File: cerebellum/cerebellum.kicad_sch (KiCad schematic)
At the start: 25 parts, among them J1 GPIO, J2 Conn_MOTA, J3 Conn_MOTB, J4 MD_POW, J5 Conn_SPI, J6 Conn_UART, J7 Conn_I2C, J8 VBUS(OUT), J9 3V3(OUT), SW1 PULLUP, SW2 PULLDOWN, SW3 SW_SPDT, U2 POLOLU_TB6612_CARRIER, U3 HC-SR04

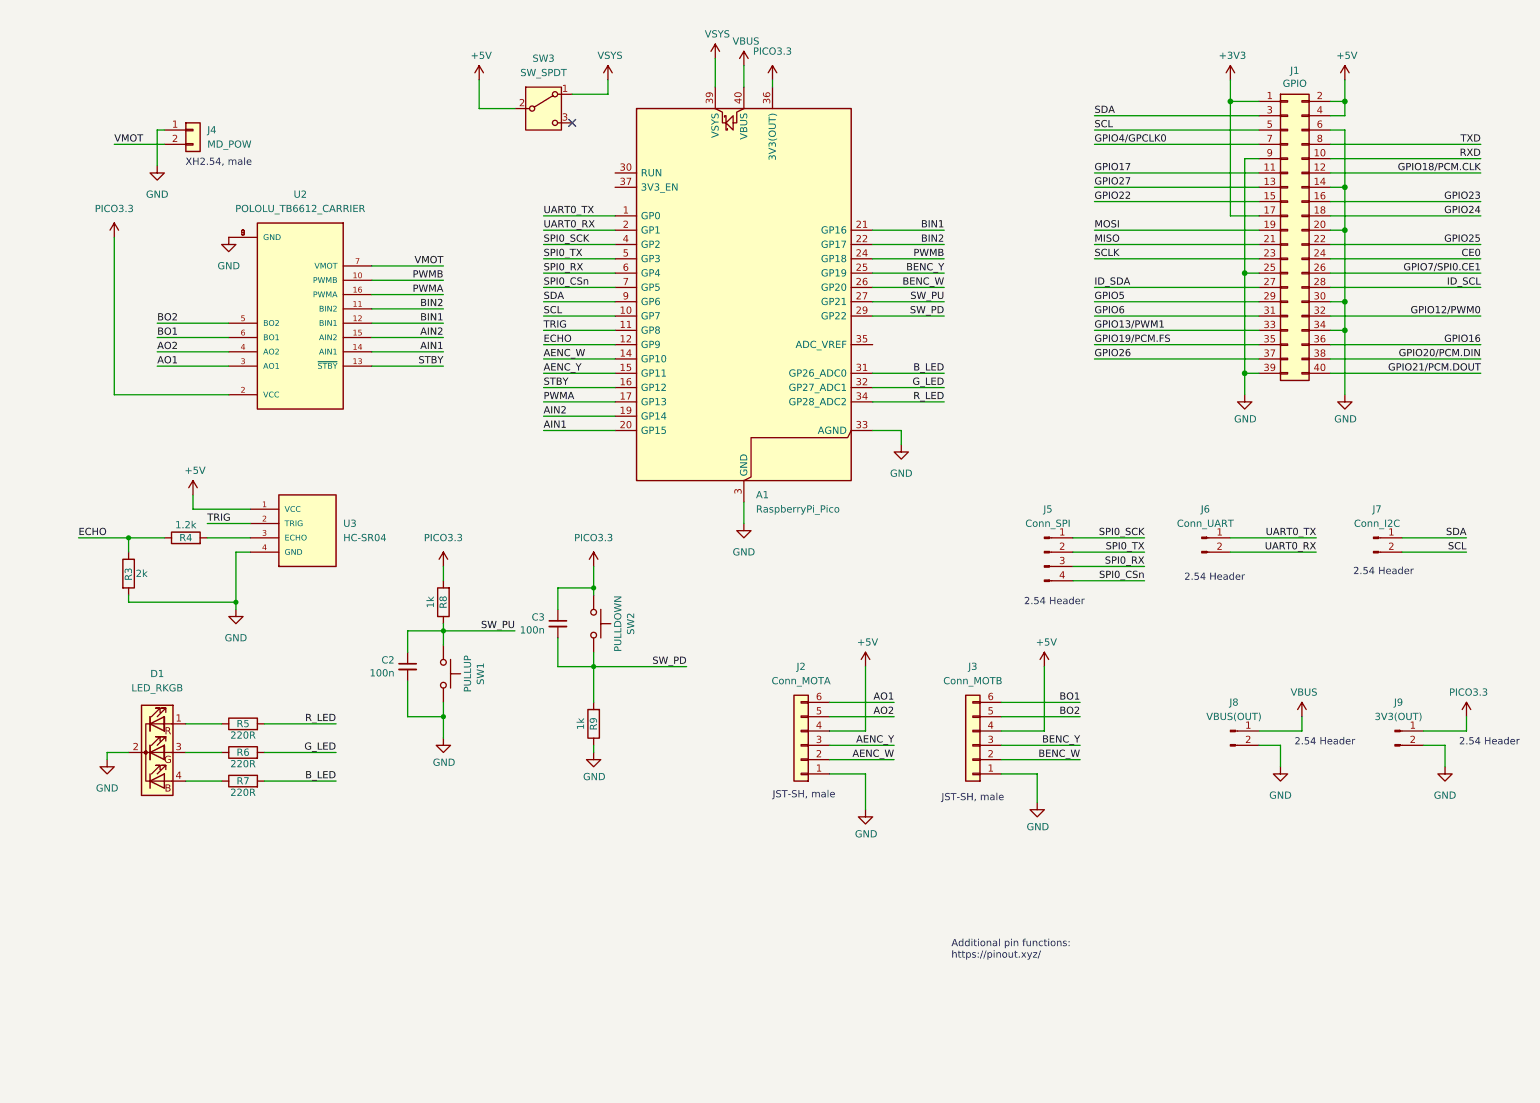
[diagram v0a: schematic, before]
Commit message: organize schematic
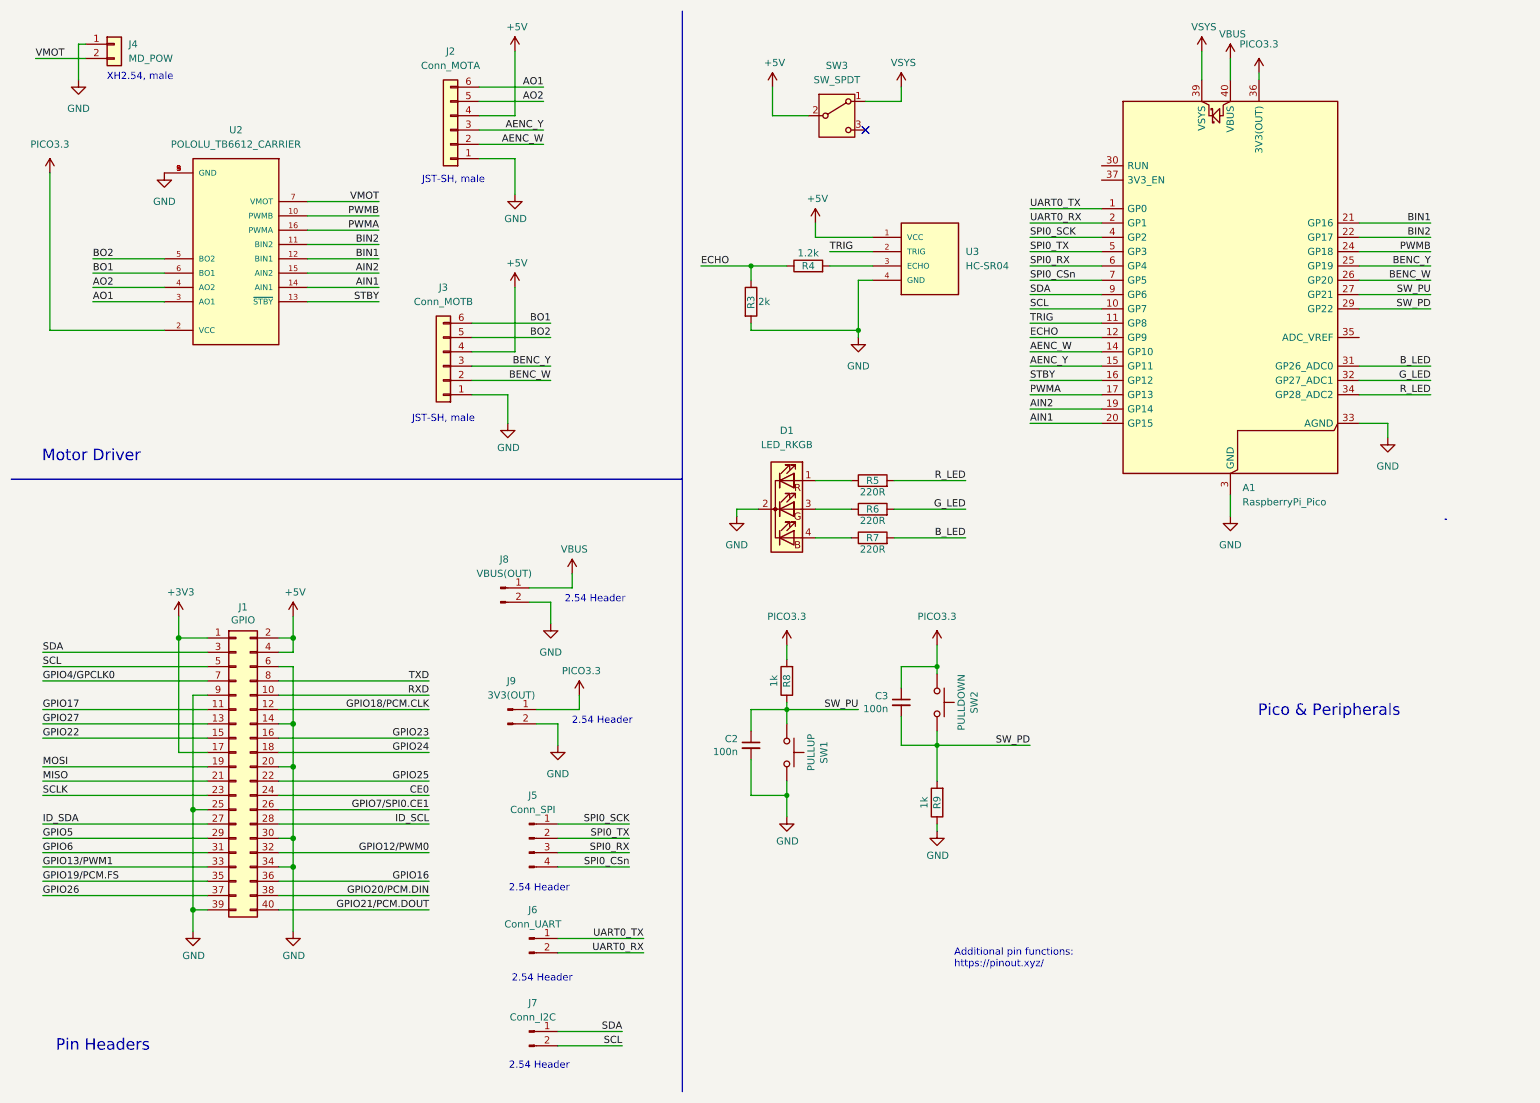
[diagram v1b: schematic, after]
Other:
- note added: "Motor Driver"
- note added: "Pico & Peripherals"
- note added: "Pin Headers"
- title: RPi Expansion for Pico and Motor Driver (The Cerebellum) -> R1R Cerebellum
- moved on the sheet: A1, C2, C3, D1, J1, J2, J3, J4, J5, J6, J7, J8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
